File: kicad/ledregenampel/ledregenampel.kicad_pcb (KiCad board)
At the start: 2 copper layers, 102 parts

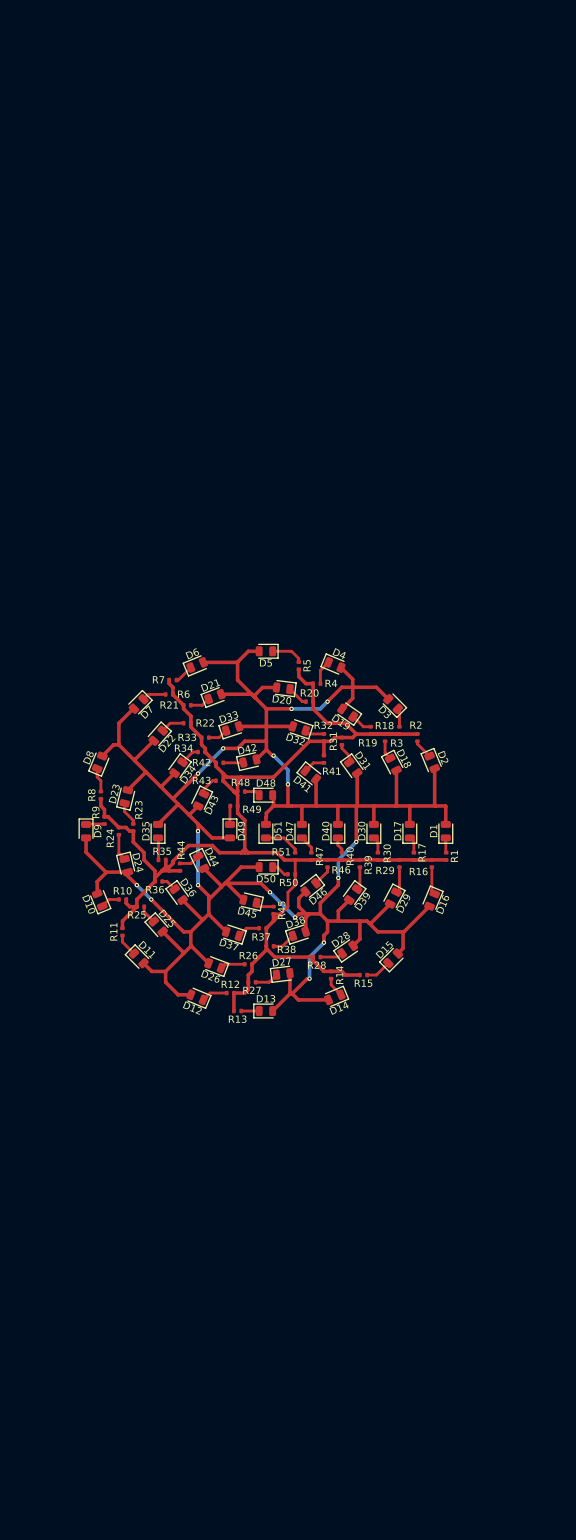
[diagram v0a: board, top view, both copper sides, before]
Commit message: lets call this RC1
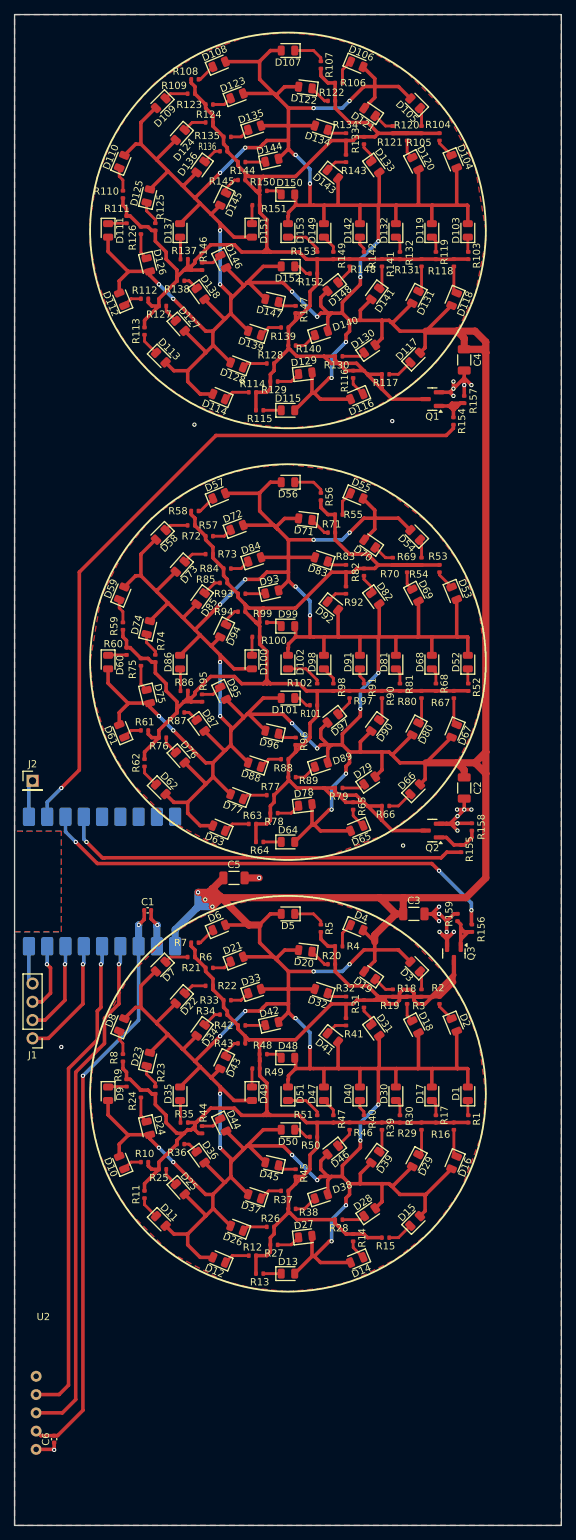
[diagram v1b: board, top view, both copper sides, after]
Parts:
- added C1: 100nF, Capacitor_SMD:C_0402_1005Metric, F.Cu at (70.5, 174.5)
- added C2: 100uF, Capacitor_SMD:C_1206_3216Metric, F.Cu at (114.5, 157.5)
- added C3: 100uF, Capacitor_SMD:C_1206_3216Metric, F.Cu at (107.5, 175.0)
- added C4: 100uF, Capacitor_SMD:C_1206_3216Metric, F.Cu at (114.5, 98.0)
- added C5: 100uF, Capacitor_SMD:C_1206_3216Metric, F.Cu at (82.5, 170.0)
- added C6: 100nF, Capacitor_SMD:C_0402_1005Metric, F.Cu at (57.5, 248.0)
- added D100: LED Y, LED_SMD:LED_0805_2012Metric, F.Cu at (85.0, 140.0)
- added D101: LED Y, LED_SMD:LED_0805_2012Metric, F.Cu at (90.0, 145.0)
- added D102: LED Y, LED_SMD:LED_0805_2012Metric, F.Cu at (90.0, 140.0)
- added D103: LED R, LED_SMD:LED_0805_2012Metric, F.Cu at (115.0, 80.0)
- added D104: LED R, LED_SMD:LED_0805_2012Metric, F.Cu at (113.1, 70.4)
- added D105: LED R, LED_SMD:LED_0805_2012Metric, F.Cu at (107.7, 62.3)
- added D106: LED R, LED_SMD:LED_0805_2012Metric, F.Cu at (99.6, 56.9)
- added D107: LED R, LED_SMD:LED_0805_2012Metric, F.Cu at (90.0, 55.0)
- added D108: LED R, LED_SMD:LED_0805_2012Metric, F.Cu at (80.4, 56.9)
- added D109: LED R, LED_SMD:LED_0805_2012Metric, F.Cu at (72.3, 62.3)
- added D110: LED R, LED_SMD:LED_0805_2012Metric, F.Cu at (66.9, 70.4)
- added D111: LED R, LED_SMD:LED_0805_2012Metric, F.Cu at (65.0, 80.0)
- added D112: LED R, LED_SMD:LED_0805_2012Metric, F.Cu at (66.9, 89.6)
- added D113: LED R, LED_SMD:LED_0805_2012Metric, F.Cu at (72.3, 97.7)
- added D114: LED R, LED_SMD:LED_0805_2012Metric, F.Cu at (80.4, 103.1)
- added D115: LED R, LED_SMD:LED_0805_2012Metric, F.Cu at (90.0, 105.0)
- added D116: LED R, LED_SMD:LED_0805_2012Metric, F.Cu at (99.6, 103.1)
- added D117: LED R, LED_SMD:LED_0805_2012Metric, F.Cu at (107.7, 97.7)
- added D118: LED R, LED_SMD:LED_0805_2012Metric, F.Cu at (113.1, 89.6)
- added D119: LED R, LED_SMD:LED_0805_2012Metric, F.Cu at (110.0, 80.0)
- added D120: LED R, LED_SMD:LED_0805_2012Metric, F.Cu at (107.7, 70.7)
- added D121: LED R, LED_SMD:LED_0805_2012Metric, F.Cu at (101.4, 63.5)
- added D122: LED R, LED_SMD:LED_0805_2012Metric, F.Cu at (92.4, 60.1)
- added D123: LED R, LED_SMD:LED_0805_2012Metric, F.Cu at (82.9, 61.3)
- added D124: LED R, LED_SMD:LED_0805_2012Metric, F.Cu at (75.0, 66.7)
- added D125: LED R, LED_SMD:LED_0805_2012Metric, F.Cu at (70.6, 75.2)
- added D126: LED R, LED_SMD:LED_0805_2012Metric, F.Cu at (70.6, 84.8)
- added D127: LED R, LED_SMD:LED_0805_2012Metric, F.Cu at (75.0, 93.3)
- added D128: LED R, LED_SMD:LED_0805_2012Metric, F.Cu at (82.9, 98.7)
- added D129: LED R, LED_SMD:LED_0805_2012Metric, F.Cu at (92.4, 99.9)
- added D130: LED R, LED_SMD:LED_0805_2012Metric, F.Cu at (101.4, 96.5)
- added D131: LED R, LED_SMD:LED_0805_2012Metric, F.Cu at (107.7, 89.3)
- added D132: LED R, LED_SMD:LED_0805_2012Metric, F.Cu at (105.0, 80.0)
- added D133: LED R, LED_SMD:LED_0805_2012Metric, F.Cu at (102.1, 71.2)
- added D134: LED R, LED_SMD:LED_0805_2012Metric, F.Cu at (94.6, 65.7)
- added D135: LED R, LED_SMD:LED_0805_2012Metric, F.Cu at (85.4, 65.7)
- added D136: LED R, LED_SMD:LED_0805_2012Metric, F.Cu at (77.9, 71.2)
- added D137: LED R, LED_SMD:LED_0805_2012Metric, F.Cu at (75.0, 80.0)
- added D138: LED R, LED_SMD:LED_0805_2012Metric, F.Cu at (77.9, 88.8)
- added D139: LED R, LED_SMD:LED_0805_2012Metric, F.Cu at (85.4, 94.3)
- added D140: LED R, LED_SMD:LED_0805_2012Metric, F.Cu at (94.6, 94.3)
- added D141: LED R, LED_SMD:LED_0805_2012Metric, F.Cu at (102.1, 88.8)
- added D142: LED R, LED_SMD:LED_0805_2012Metric, F.Cu at (100.0, 80.0)
- added D143: LED R, LED_SMD:LED_0805_2012Metric, F.Cu at (96.2, 72.2)
- added D144: LED R, LED_SMD:LED_0805_2012Metric, F.Cu at (87.8, 70.3)
- added D145: LED R, LED_SMD:LED_0805_2012Metric, F.Cu at (81.0, 75.7)
- added D146: LED R, LED_SMD:LED_0805_2012Metric, F.Cu at (81.0, 84.3)
- added D147: LED R, LED_SMD:LED_0805_2012Metric, F.Cu at (87.8, 89.7)
- added D148: LED R, LED_SMD:LED_0805_2012Metric, F.Cu at (96.2, 87.8)
- added D149: LED R, LED_SMD:LED_0805_2012Metric, F.Cu at (95.0, 80.0)
- added D150: LED R, LED_SMD:LED_0805_2012Metric, F.Cu at (90.0, 75.0)
- added D151: LED R, LED_SMD:LED_0805_2012Metric, F.Cu at (85.0, 80.0)
- added D152: LED R, LED_SMD:LED_0805_2012Metric, F.Cu at (90.0, 85.0)
- added D153: LED R, LED_SMD:LED_0805_2012Metric, F.Cu at (90.0, 80.0)
- added D52: LED Y, LED_SMD:LED_0805_2012Metric, F.Cu at (115.0, 140.0)
- added D53: LED Y, LED_SMD:LED_0805_2012Metric, F.Cu at (113.1, 130.4)
- added D54: LED Y, LED_SMD:LED_0805_2012Metric, F.Cu at (107.7, 122.3)
- added D55: LED Y, LED_SMD:LED_0805_2012Metric, F.Cu at (99.6, 116.9)
- added D56: LED Y, LED_SMD:LED_0805_2012Metric, F.Cu at (90.0, 115.0)
- added D57: LED Y, LED_SMD:LED_0805_2012Metric, F.Cu at (80.4, 116.9)
- added D58: LED Y, LED_SMD:LED_0805_2012Metric, F.Cu at (72.3, 122.3)
- added D59: LED Y, LED_SMD:LED_0805_2012Metric, F.Cu at (66.9, 130.4)
- added D60: LED Y, LED_SMD:LED_0805_2012Metric, F.Cu at (65.0, 140.0)
- added D61: LED Y, LED_SMD:LED_0805_2012Metric, F.Cu at (66.9, 149.6)
- added D62: LED Y, LED_SMD:LED_0805_2012Metric, F.Cu at (72.3, 157.7)
- added D63: LED Y, LED_SMD:LED_0805_2012Metric, F.Cu at (80.4, 163.1)
- added D64: LED Y, LED_SMD:LED_0805_2012Metric, F.Cu at (90.0, 165.0)
- added D65: LED Y, LED_SMD:LED_0805_2012Metric, F.Cu at (99.6, 163.1)
- added D66: LED Y, LED_SMD:LED_0805_2012Metric, F.Cu at (107.7, 157.7)
- added D67: LED Y, LED_SMD:LED_0805_2012Metric, F.Cu at (113.1, 149.6)
- added D68: LED Y, LED_SMD:LED_0805_2012Metric, F.Cu at (110.0, 140.0)
- added D69: LED Y, LED_SMD:LED_0805_2012Metric, F.Cu at (107.7, 130.7)
- added D70: LED Y, LED_SMD:LED_0805_2012Metric, F.Cu at (101.4, 123.5)
- added D71: LED Y, LED_SMD:LED_0805_2012Metric, F.Cu at (92.4, 120.1)
- added D72: LED Y, LED_SMD:LED_0805_2012Metric, F.Cu at (82.9, 121.3)
- added D73: LED Y, LED_SMD:LED_0805_2012Metric, F.Cu at (75.0, 126.7)
- added D74: LED Y, LED_SMD:LED_0805_2012Metric, F.Cu at (70.6, 135.2)
- added D75: LED Y, LED_SMD:LED_0805_2012Metric, F.Cu at (70.6, 144.8)
- added D76: LED Y, LED_SMD:LED_0805_2012Metric, F.Cu at (75.0, 153.3)
- added D77: LED Y, LED_SMD:LED_0805_2012Metric, F.Cu at (82.9, 158.7)
- added D78: LED Y, LED_SMD:LED_0805_2012Metric, F.Cu at (92.4, 159.9)
- added D79: LED Y, LED_SMD:LED_0805_2012Metric, F.Cu at (101.4, 156.5)
- added D80: LED Y, LED_SMD:LED_0805_2012Metric, F.Cu at (107.7, 149.3)
- added D81: LED Y, LED_SMD:LED_0805_2012Metric, F.Cu at (105.0, 140.0)
- added D82: LED Y, LED_SMD:LED_0805_2012Metric, F.Cu at (102.1, 131.2)
- added D83: LED Y, LED_SMD:LED_0805_2012Metric, F.Cu at (94.6, 125.7)
- added D84: LED Y, LED_SMD:LED_0805_2012Metric, F.Cu at (85.4, 125.7)
- added D85: LED Y, LED_SMD:LED_0805_2012Metric, F.Cu at (77.9, 131.2)
- added D86: LED Y, LED_SMD:LED_0805_2012Metric, F.Cu at (75.0, 140.0)
- added D87: LED Y, LED_SMD:LED_0805_2012Metric, F.Cu at (77.9, 148.8)
- added D88: LED Y, LED_SMD:LED_0805_2012Metric, F.Cu at (85.4, 154.3)
- added D89: LED Y, LED_SMD:LED_0805_2012Metric, F.Cu at (94.6, 154.3)
- added D90: LED Y, LED_SMD:LED_0805_2012Metric, F.Cu at (102.1, 148.8)
- added D91: LED Y, LED_SMD:LED_0805_2012Metric, F.Cu at (100.0, 140.0)
- added D92: LED Y, LED_SMD:LED_0805_2012Metric, F.Cu at (96.2, 132.2)
- added D93: LED Y, LED_SMD:LED_0805_2012Metric, F.Cu at (87.8, 130.3)
- added D94: LED Y, LED_SMD:LED_0805_2012Metric, F.Cu at (81.0, 135.7)
- added D95: LED Y, LED_SMD:LED_0805_2012Metric, F.Cu at (81.0, 144.3)
- added D96: LED Y, LED_SMD:LED_0805_2012Metric, F.Cu at (87.8, 149.7)
- added D97: LED Y, LED_SMD:LED_0805_2012Metric, F.Cu at (96.2, 147.8)
- added D98: LED Y, LED_SMD:LED_0805_2012Metric, F.Cu at (95.0, 140.0)
- added D99: LED Y, LED_SMD:LED_0805_2012Metric, F.Cu at (90.0, 135.0)
- added J1: Exp-Conn1, Connector_PinHeader_2.54mm:PinHeader_1x04_P2.54mm_Vertical, F.Cu at (54.5, 192.3)
- added J2: Exp-Conn2, Connector_PinHeader_2.54mm:PinHeader_1x01_P2.54mm_Vertical, F.Cu at (54.5, 156.5)
- added Q1: AO3400A, Package_TO_SOT_SMD:SOT-23, F.Cu at (110.1, 103.5)
- added Q2: AO3400A, Package_TO_SOT_SMD:SOT-23, F.Cu at (110.1, 163.4)
- added Q3: AO3400A, Package_TO_SOT_SMD:SOT-23, F.Cu at (113.1, 180.5)
- added R100: 150Ω, foxisfrickellibrary:R_0402_modsilkscreen, F.Cu at (85.6, 136.5)
- added R101: 150Ω, foxisfrickellibrary:R_0402_modsilkscreen, F.Cu at (93.6, 146.0)
- added R102: 150Ω, foxisfrickellibrary:R_0402_modsilkscreen, F.Cu at (94.1, 143.5)
- added R103: 150Ω, foxisfrickellibrary:R_0402_modsilkscreen, F.Cu at (115.1, 83.5)
- added R104: 150Ω, foxisfrickellibrary:R_0402_modsilkscreen, F.Cu at (111.1, 67.0)
- added R105: 150Ω, foxisfrickellibrary:R_0402_modsilkscreen, F.Cu at (108.6, 66.0)
- added R106: 150Ω, foxisfrickellibrary:R_0402_modsilkscreen, F.Cu at (97.1, 59.5)
- added R107: 150Ω, foxisfrickellibrary:R_0402_modsilkscreen, F.Cu at (94.6, 57.0)
- added R108: 150Ω, foxisfrickellibrary:R_0402_modsilkscreen, F.Cu at (77.1, 59.0)
- added R109: 150Ω, foxisfrickellibrary:R_0402_modsilkscreen, F.Cu at (76.6, 61.0)
- added R110: 150Ω, foxisfrickellibrary:R_0402_modsilkscreen, F.Cu at (67.1, 75.0)
- added R111: 150Ω, foxisfrickellibrary:R_0402_modsilkscreen, F.Cu at (67.6, 78.5)
- added R112: 150Ω, foxisfrickellibrary:R_0402_modsilkscreen, F.Cu at (70.1, 89.5)
- added R113: 150Ω, foxisfrickellibrary:R_0402_modsilkscreen, F.Cu at (70.1, 94.0)
- added R114: 150Ω, foxisfrickellibrary:R_0402_modsilkscreen, F.Cu at (85.1, 102.5)
- added R115: 150Ω, foxisfrickellibrary:R_0402_modsilkscreen, F.Cu at (86.1, 105.0)
- added R116: 150Ω, foxisfrickellibrary:R_0402_modsilkscreen, F.Cu at (99.1, 100.0)
- added R117: 150Ω, foxisfrickellibrary:R_0402_modsilkscreen, F.Cu at (103.6, 100.0)
- added R118: 150Ω, foxisfrickellibrary:R_0402_modsilkscreen, F.Cu at (113.1, 84.5)
- added R119: 150Ω, foxisfrickellibrary:R_0402_modsilkscreen, F.Cu at (110.6, 83.5)
- added R120: 150Ω, foxisfrickellibrary:R_0402_modsilkscreen, F.Cu at (106.6, 67.0)
- added R121: 150Ω, foxisfrickellibrary:R_0402_modsilkscreen, F.Cu at (104.6, 66.0)
- added R122: 150Ω, foxisfrickellibrary:R_0402_modsilkscreen, F.Cu at (96.1, 62.0)
- added R123: 150Ω, foxisfrickellibrary:R_0402_modsilkscreen, F.Cu at (79.1, 62.5)
- added R124: 150Ω, foxisfrickellibrary:R_0402_modsilkscreen, F.Cu at (79.1, 65.0)
- added R125: 150Ω, foxisfrickellibrary:R_0402_modsilkscreen, F.Cu at (71.6, 79.5)
- added R126: 150Ω, foxisfrickellibrary:R_0402_modsilkscreen, F.Cu at (69.6, 80.0)
- added R127: 150Ω, foxisfrickellibrary:R_0402_modsilkscreen, F.Cu at (72.6, 90.5)
- added R128: 150Ω, foxisfrickellibrary:R_0402_modsilkscreen, F.Cu at (87.6, 98.5)
- added R129: 150Ω, foxisfrickellibrary:R_0402_modsilkscreen, F.Cu at (88.1, 101.0)
- added R130: 150Ω, foxisfrickellibrary:R_0402_modsilkscreen, F.Cu at (97.1, 97.5)
- added R131: 150Ω, foxisfrickellibrary:R_0402_modsilkscreen, F.Cu at (108.6, 84.5)
- added R132: 150Ω, foxisfrickellibrary:R_0402_modsilkscreen, F.Cu at (105.6, 83.5)
- added R133: 150Ω, foxisfrickellibrary:R_0402_modsilkscreen, F.Cu at (100.6, 67.5)
- added R134: 150Ω, foxisfrickellibrary:R_0402_modsilkscreen, F.Cu at (98.1, 67.0)
- added R135: 150Ω, foxisfrickellibrary:R_0402_modsilkscreen, F.Cu at (81.6, 67.0)
- added R136: 150Ω, foxisfrickellibrary:R_0402_modsilkscreen, F.Cu at (81.1, 69.0)
- added R137: 150Ω, foxisfrickellibrary:R_0402_modsilkscreen, F.Cu at (75.6, 84.0)
- added R138: 150Ω, foxisfrickellibrary:R_0402_modsilkscreen, F.Cu at (75.1, 87.0)
- added R139: 150Ω, foxisfrickellibrary:R_0402_modsilkscreen, F.Cu at (89.6, 93.5)
- added R140: 150Ω, foxisfrickellibrary:R_0402_modsilkscreen, F.Cu at (90.6, 96.0)
- added R141: 150Ω, foxisfrickellibrary:R_0402_modsilkscreen, F.Cu at (103.1, 84.5)
- added R142: 150Ω, foxisfrickellibrary:R_0402_modsilkscreen, F.Cu at (100.6, 83.5)
- added R143: 150Ω, foxisfrickellibrary:R_0402_modsilkscreen, F.Cu at (98.1, 70.0)
- added R144: 150Ω, foxisfrickellibrary:R_0402_modsilkscreen, F.Cu at (83.6, 70.5)
- added R145: 150Ω, foxisfrickellibrary:R_0402_modsilkscreen, F.Cu at (83.6, 73.0)
- added R146: 150Ω, foxisfrickellibrary:R_0402_modsilkscreen, F.Cu at (78.1, 85.0)
- added R147: 150Ω, foxisfrickellibrary:R_0402_modsilkscreen, F.Cu at (91.1, 91.0)
- added R148: 150Ω, foxisfrickellibrary:R_0402_modsilkscreen, F.Cu at (98.6, 84.5)
- added R149: 150Ω, foxisfrickellibrary:R_0402_modsilkscreen, F.Cu at (96.3, 83.5)
- added R150: 150Ω, foxisfrickellibrary:R_0402_modsilkscreen, F.Cu at (86.6, 74.5)
- added R151: 150Ω, foxisfrickellibrary:R_0402_modsilkscreen, F.Cu at (85.6, 76.5)
- added R152: 150Ω, foxisfrickellibrary:R_0402_modsilkscreen, F.Cu at (93.6, 86.0)
- added R153: 150Ω, foxisfrickellibrary:R_0402_modsilkscreen, F.Cu at (94.1, 83.5)
- added R154: 33Ω, foxisfrickellibrary:R_0402_modsilkscreen, F.Cu at (113.0, 106.5)
- added R155: 33Ω, foxisfrickellibrary:R_0402_modsilkscreen, F.Cu at (114.1, 165.9)
- added R156: 33Ω, foxisfrickellibrary:R_0402_modsilkscreen, F.Cu at (115.6, 177.0)
- added R157: 1MΩ, foxisfrickellibrary:R_0402_modsilkscreen, F.Cu at (114.5, 103.5)
- added R158: 1MΩ, foxisfrickellibrary:R_0402_modsilkscreen, F.Cu at (115.6, 162.9)
- added R159: 1MΩ, foxisfrickellibrary:R_0402_modsilkscreen, F.Cu at (113.6, 175.5)
- added R52: 150Ω, foxisfrickellibrary:R_0402_modsilkscreen, F.Cu at (115.1, 143.5)
- added R53: 150Ω, foxisfrickellibrary:R_0402_modsilkscreen, F.Cu at (111.1, 127.0)
- added R54: 150Ω, foxisfrickellibrary:R_0402_modsilkscreen, F.Cu at (108.6, 126.0)
- added R55: 150Ω, foxisfrickellibrary:R_0402_modsilkscreen, F.Cu at (97.1, 119.5)
- added R56: 150Ω, foxisfrickellibrary:R_0402_modsilkscreen, F.Cu at (94.6, 117.0)
- added R57: 150Ω, foxisfrickellibrary:R_0402_modsilkscreen, F.Cu at (77.1, 119.0)
- added R58: 150Ω, foxisfrickellibrary:R_0402_modsilkscreen, F.Cu at (76.6, 121.0)
- added R59: 150Ω, foxisfrickellibrary:R_0402_modsilkscreen, F.Cu at (67.1, 135.0)
- added R60: 150Ω, foxisfrickellibrary:R_0402_modsilkscreen, F.Cu at (67.6, 138.5)
- added R61: 150Ω, foxisfrickellibrary:R_0402_modsilkscreen, F.Cu at (70.1, 149.5)
- added R62: 150Ω, foxisfrickellibrary:R_0402_modsilkscreen, F.Cu at (70.1, 154.0)
- added R63: 150Ω, foxisfrickellibrary:R_0402_modsilkscreen, F.Cu at (85.1, 162.5)
- added R64: 150Ω, foxisfrickellibrary:R_0402_modsilkscreen, F.Cu at (86.1, 165.0)
- added R65: 150Ω, foxisfrickellibrary:R_0402_modsilkscreen, F.Cu at (99.1, 160.0)
- added R66: 150Ω, foxisfrickellibrary:R_0402_modsilkscreen, F.Cu at (103.6, 160.0)
- added R67: 150Ω, foxisfrickellibrary:R_0402_modsilkscreen, F.Cu at (113.1, 144.5)
- added R68: 150Ω, foxisfrickellibrary:R_0402_modsilkscreen, F.Cu at (110.6, 143.5)
- added R69: 150Ω, foxisfrickellibrary:R_0402_modsilkscreen, F.Cu at (106.6, 127.0)
- added R70: 150Ω, foxisfrickellibrary:R_0402_modsilkscreen, F.Cu at (104.6, 126.0)
- added R71: 150Ω, foxisfrickellibrary:R_0402_modsilkscreen, F.Cu at (96.1, 122.0)
- added R72: 150Ω, foxisfrickellibrary:R_0402_modsilkscreen, F.Cu at (79.1, 122.5)
- added R73: 150Ω, foxisfrickellibrary:R_0402_modsilkscreen, F.Cu at (79.1, 125.0)
- added R74: 150Ω, foxisfrickellibrary:R_0402_modsilkscreen, F.Cu at (71.6, 139.5)
- added R75: 150Ω, foxisfrickellibrary:R_0402_modsilkscreen, F.Cu at (69.6, 140.0)
- added R76: 150Ω, foxisfrickellibrary:R_0402_modsilkscreen, F.Cu at (72.6, 150.5)
- added R77: 150Ω, foxisfrickellibrary:R_0402_modsilkscreen, F.Cu at (87.6, 158.5)
- added R78: 150Ω, foxisfrickellibrary:R_0402_modsilkscreen, F.Cu at (88.1, 161.0)
- added R79: 150Ω, foxisfrickellibrary:R_0402_modsilkscreen, F.Cu at (97.1, 157.5)
- added R80: 150Ω, foxisfrickellibrary:R_0402_modsilkscreen, F.Cu at (108.6, 144.5)
- added R81: 150Ω, foxisfrickellibrary:R_0402_modsilkscreen, F.Cu at (105.6, 143.5)
- added R82: 150Ω, foxisfrickellibrary:R_0402_modsilkscreen, F.Cu at (100.6, 127.5)
- added R83: 150Ω, foxisfrickellibrary:R_0402_modsilkscreen, F.Cu at (98.1, 127.0)
- added R84: 150Ω, foxisfrickellibrary:R_0402_modsilkscreen, F.Cu at (81.6, 127.0)
- added R85: 150Ω, foxisfrickellibrary:R_0402_modsilkscreen, F.Cu at (81.1, 129.0)
- added R86: 150Ω, foxisfrickellibrary:R_0402_modsilkscreen, F.Cu at (75.6, 144.0)
- added R87: 150Ω, foxisfrickellibrary:R_0402_modsilkscreen, F.Cu at (75.1, 147.0)
- added R88: 150Ω, foxisfrickellibrary:R_0402_modsilkscreen, F.Cu at (89.6, 153.5)
- added R89: 150Ω, foxisfrickellibrary:R_0402_modsilkscreen, F.Cu at (90.6, 156.0)
- added R90: 150Ω, foxisfrickellibrary:R_0402_modsilkscreen, F.Cu at (103.1, 144.5)
- added R91: 150Ω, foxisfrickellibrary:R_0402_modsilkscreen, F.Cu at (100.6, 143.5)
- added R92: 150Ω, foxisfrickellibrary:R_0402_modsilkscreen, F.Cu at (98.1, 130.0)
- added R93: 150Ω, foxisfrickellibrary:R_0402_modsilkscreen, F.Cu at (83.6, 130.5)
- added R94: 150Ω, foxisfrickellibrary:R_0402_modsilkscreen, F.Cu at (83.6, 133.0)
- added R95: 150Ω, foxisfrickellibrary:R_0402_modsilkscreen, F.Cu at (78.1, 145.0)
- added R96: 150Ω, foxisfrickellibrary:R_0402_modsilkscreen, F.Cu at (91.1, 151.0)
- added R97: 150Ω, foxisfrickellibrary:R_0402_modsilkscreen, F.Cu at (98.6, 144.5)
- added R98: 150Ω, foxisfrickellibrary:R_0402_modsilkscreen, F.Cu at (96.3, 143.5)
- added R99: 150Ω, foxisfrickellibrary:R_0402_modsilkscreen, F.Cu at (86.6, 134.5)
- added U1: Waveshare ESP32-C3 Mini, foxisfrickellibrary:Waveshare_ESP32-C3_Mini, B.Cu at (74.3, 170.5)
- added U2: ~, foxisfrickellibrary:OLED-2.08-inch, F.Cu at (53.5, 232.0)
- R1, R10, R11, R12, R13, R14, R15, R16, R17, R18, R19, R2, R20, R21, R22, R23, R24, R25, R26, R27, R28, R29, R3, R30, R31, R32, R33, R34, R35, R36, R37, R38, R39, R4, R40, R41, R42, R43, R44, R45, R46, R47, R48, R49, R5, R50, R51, R6, R7, R8, R9: value 110 -> 120Ω
- moved D1 36.6 mm to (115.0, 200.0)
- moved D10 36.6 mm to (66.9, 209.6)
- moved D11 36.6 mm to (72.3, 217.7)
- moved D12 36.6 mm to (80.4, 223.1)
- moved D13 36.6 mm to (90.0, 225.0)
- moved D14 36.6 mm to (99.6, 223.1)
- moved D15 36.6 mm to (107.7, 217.7)
- moved D16 36.6 mm to (113.1, 209.6)
- moved D17 36.6 mm to (110.0, 200.0)
- moved D18 36.6 mm to (107.7, 190.7)
- moved D19 36.6 mm to (101.4, 183.5)
- moved D2 36.6 mm to (113.1, 190.4)
- moved D20 36.6 mm to (92.4, 180.1)
- moved D21 36.6 mm to (82.9, 181.3)
- moved D22 36.6 mm to (75.0, 186.7)
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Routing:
- net +5V: track 382.0 -> 1331.7 mm, vias 16 -> 51
- net /R2MOSFET: track 0.00 -> 218.6 mm
- net /Y2MOSFET: track 0.00 -> 218.5 mm
- net Net-(U1-GP7): track 0.00 -> 96.6 mm, vias 0 -> 1
- net +3V3: track 0.00 -> 81.2 mm, vias 0 -> 2
- net Net-(U1-GP0): track 0.00 -> 71.8 mm, vias 0 -> 1
- net Net-(U1-GP1): track 0.00 -> 68.0 mm, vias 0 -> 1
- net Net-(U1-GP8): track 0.00 -> 65.6 mm, vias 0 -> 3
- net Net-(U1-GP9): track 0.00 -> 57.0 mm, vias 0 -> 1
- net GND: track 0.00 -> 48.9 mm, vias 0 -> 24
- net /G2MOSFET: track 200.6 -> 219.0 mm
- net Net-(J1-Pin_1): track 0.00 -> 17.0 mm, vias 0 -> 1
- net Net-(J1-Pin_2): track 0.00 -> 13.2 mm, vias 0 -> 1
- net Net-(J1-Pin_3): track 0.00 -> 9.73 mm, vias 0 -> 1
- net Net-(Q1-G): track 0.00 -> 8.54 mm
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- added copper zone on F.Cu, net +5V
- added copper zone on B.Cu, net GND
- added copper zone on F.Cu, net GND
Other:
- board outline added: 76 x 210 mm
